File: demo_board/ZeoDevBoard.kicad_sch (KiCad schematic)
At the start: 0 parts

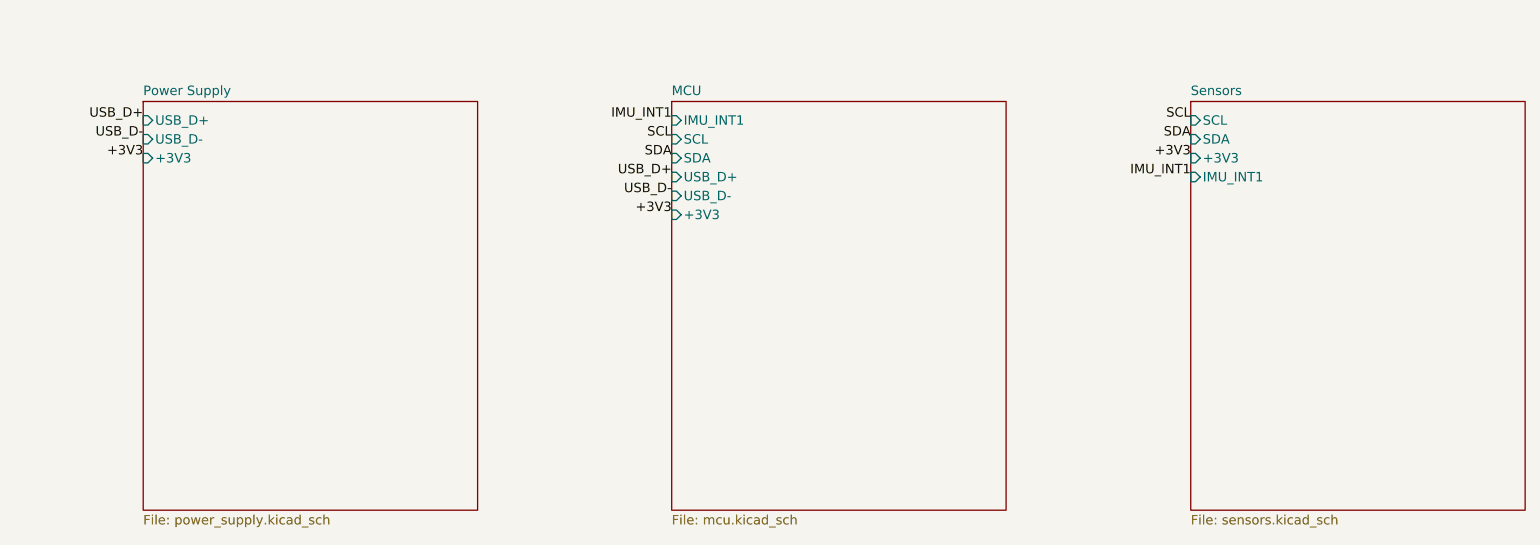
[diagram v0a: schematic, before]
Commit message: new demo board
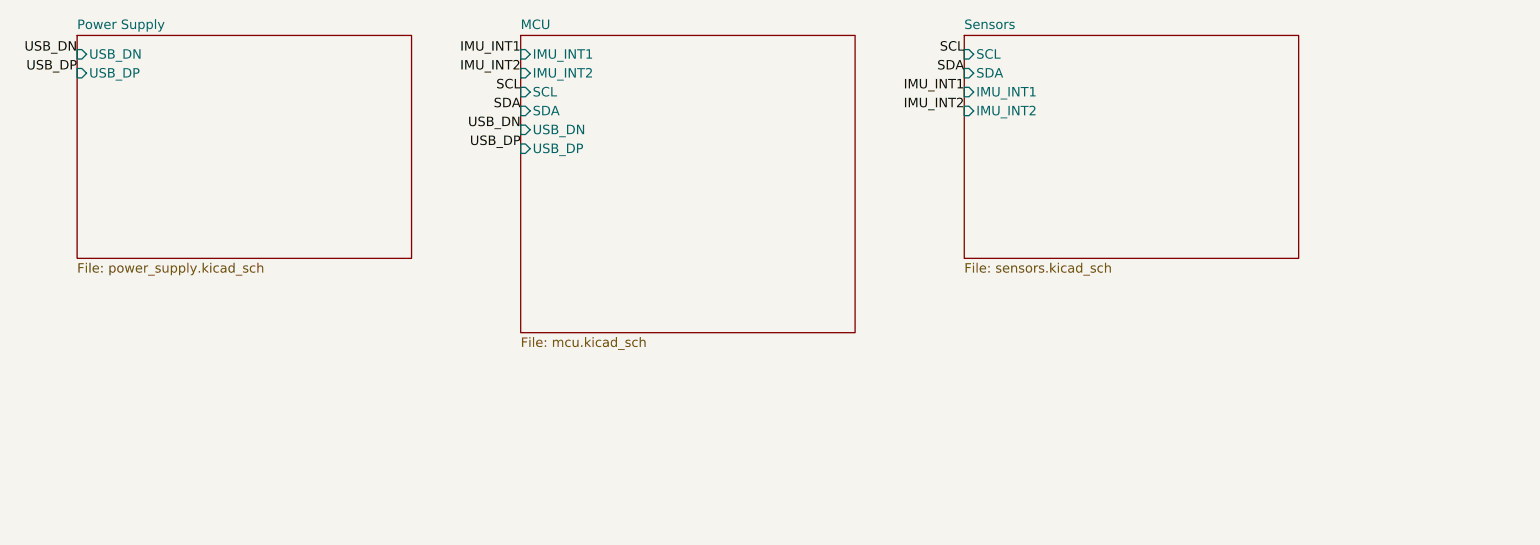
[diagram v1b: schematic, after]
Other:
- sheet MCU ports: added IMU_INT2, USB_DN, USB_DP; removed +3V3, USB_D+, USB_D-
- sheet Power Supply ports: added USB_DN, USB_DP; removed +3V3, USB_D+, USB_D-
- sheet Sensors ports: added IMU_INT2; removed +3V3
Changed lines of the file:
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@@
 	(generator_version "10.0")
 	(paper "A4")
-	(label "USB_D-"
-		(at 39.37 44.45 180)
-		(effects
-			(font
-				(size 1.27 1.27)
-				(line_spacing 0)
-			)
-			(justify right bottom)
-		)
-	)
-	(label "+3V3"
-		(at 110.49 54.61 180)
+	(label "USB_DP"
+		(at 30.48 35.56 180)
+		(effects
+			(font
+				(size 1.27 1.27)
+				(line_spacing 0)
+			)
+			(justify right bottom)
+		)
+	)
+	(label "IMU_INT2"
+		(at 90.17 35.56 180)
+		(effects
+			(font
+				(size 1.27 1.27)
+				(line_spacing 0)
+			)
+			(justify right bottom)
+		)
+	)
+	(label "USB_DN"
+		(at 30.48 33.02 180)
+		(effects
+			(font
+				(size 1.27 1.27)
+				(line_spacing 0)
+			)
+			(justify right bottom)
+		)
+	)
+	(label "USB_DP"
+		(at 90.17 45.72 180)
+		(effects
+			(font
+				(size 1.27 1.27)
+				(line_spacing 0)
+			)
+			(justify right bottom)
+		)
+	)
+	(label "IMU_INT1"
+		(at 149.86 38.1 180)
+		(effects
+			(font
+				(size 1.27 1.27)
+				(line_spacing 0)
+			)
+			(justify right bottom)
+		)
+	)
+	(label "USB_DN"
+		(at 90.17 43.18 180)
+		(effects
+			(font
+				(size 1.27 1.27)
+				(line_spacing 0)
+			)
+			(justify right bottom)
+		)
+	)
+	(label "IMU_INT2"
+		(at 149.86 40.64 180)
 		(effects
 			(font
@@
 	)
 	(label "SCL"
-		(at 110.49 44.45 180)
-		(effects
-			(font
-				(size 1.27 1.27)
-				(line_spacing 0)
-			)
-			(justify right bottom)
-		)
-	)
-	(label "USB_D+"
-		(at 39.37 41.91 180)
+		(at 149.86 33.02 180)
+		(effects
+			(font
+				(size 1.27 1.27)
+				(line_spacing 0)
+			)
+			(justify right bottom)
+		)
+	)
+	(label "SCL"
+		(at 90.17 38.1 180)
+		(effects
+			(font
+				(size 1.27 1.27)
+				(line_spacing 0)
+			)
+			(justify right bottom)
+		)
+	)
+	(label "SDA"
+		(at 90.17 40.64 180)
 		(effects
 			(font
@@
 	)
 	(label "IMU_INT1"
-		(at 180.34 49.53 180)
+		(at 90.17 33.02 180)
 		(effects
 			(font
@@
 	)
 	(label "SDA"
-		(at 180.34 44.45 180)
-		(effects
-			(font
-				(size 1.27 1.27)
-				(line_spacing 0)
-			)
-			(justify right bottom)
-		)
-	)
-	(label "+3V3"
-		(at 39.37 46.99 180)
-		(effects
-			(font
-				(size 1.27 1.27)
-				(line_spacing 0)
-			)
-			(justify right bottom)
-		)
-	)
-	(label "+3V3"
-		(at 180.34 46.99 180)
-		(effects
-			(font
-				(size 1.27 1.27)
-				(line_spacing 0)
-			)
-			(justify right bottom)
-		)
-	)
-	(label "SCL"
-		(at 180.34 41.91 180)
-		(effects
-			(font
-				(size 1.27 1.27)
-				(line_spacing 0)
-			)
-			(justify right bottom)
-		)
-	)
-	(label "USB_D+"
-		(at 110.49 49.53 180)
-		(effects
-			(font
-				(size 1.27 1.27)
-				(line_spacing 0)
-			)
-			(justify right bottom)
-		)
-	)
-	(label "SDA"
-		(at 110.49 46.99 180)
-		(effects
-			(font
-				(size 1.27 1.27)
-				(line_spacing 0)
-			)
-			(justify right bottom)
-		)
-	)
-	(label "USB_D-"
-		(at 110.49 52.07 180)
-		(effects
-			(font
-				(size 1.27 1.27)
-				(line_spacing 0)
-			)
-			(justify right bottom)
-		)
-	)
-	(label "IMU_INT1"
-		(at 110.49 41.91 180)
+		(at 149.86 35.56 180)
 		(effects
 			(font
@@
 	)
 	(sheet
-		(at 180.34 39.37)
-		(size 45 55)
+		(at 149.86 30.48)
+		(size 45 30)
 		(exclude_from_sim no)
 		(in_bom yes)
@@
 		)
 		(property "Sheetname" "Sensors"
-			(at 180.34 38.6584 0)
+			(at 149.86 29.7684 0)
 			(show_name no)
 			(do_not_autoplace no)
@@
 		)
 		(property "Sheetfile" "sensors.kicad_sch"
-			(at 180.34 94.9546 0)
+			(at 149.86 61.0646 0)
 			(show_name no)
 			(do_not_autoplace no)
@@
 		)
 		(pin "SCL" input
-			(at 180.34 41.91 180)
+			(at 149.86 33.02 180)
 			(effects
 				(font
@@
 		)
 		(pin "SDA" input
-			(at 180.34 44.45 180)
-			(effects
-				(font
-					(size 1.27 1.27)
-				)
-				(justify left)
-			)
-		)
-		(pin "+3V3" input
-			(at 180.34 46.99 180)
+			(at 149.86 35.56 180)
 			(effects
 				(font
@@
 		)
 		(pin "IMU_INT1" input
-			(at 180.34 49.53 180)
+			(at 149.86 38.1 180)
+			(effects
+				(font
+					(size 1.27 1.27)
+				)
+				(justify left)
+			)
+		)
+		(pin "IMU_INT2" input
+			(at 149.86 40.64 180)
 			(effects
 				(font
@@
 	)
 	(sheet
-		(at 110.49 39.37)
-		(size 45 55)
+		(at 30.48 30.48)
+		(size 45 30)
 		(exclude_from_sim no)
 		(in_bom yes)
@@
 			(color 0 0 0 0)
 		)
-		(property "Sheetname" "MCU"
-			(at 110.49 38.6584 0)
+		(property "Sheetname" "Power Supply"
+			(at 30.48 29.7684 0)
 			(show_name no)
 			(do_not_autoplace no)
@@
 			)
 		)
-		(property "Sheetfile" "mcu.kicad_sch"
-			(at 110.49 94.9546 0)
+		(property "Sheetfile" "power_supply.kicad_sch"
+			(at 30.48 61.0646 0)
 			(show_name no)
 			(do_not_autoplace no)
@@
 			)
 		)
-		(pin "IMU_INT1" input
-			(at 110.49 41.91 180)
-			(effects
-				(font
-					(size 1.27 1.27)
-				)
-				(justify left)
-			)
-		)
-		(pin "SCL" input
-			(at 110.49 44.45 180)
-			(effects
-				(font
-					(size 1.27 1.27)
-				)
-				(justify left)
-			)
-		)
-		(pin "SDA" input
-			(at 110.49 46.99 180)
-			(effects
-				(font
-					(size 1.27 1.27)
-				)
-				(justify left)
-			)
-		)
-		(pin "USB_D+" input
-			(at 110.49 49.53 180)
-			(effects
-				(font
-					(size 1.27 1.27)
-				)
-				(justify left)
-			)
-		)
-		(pin "USB_D-" input
-			(at 110.49 52.07 180)
-			(effects
-				(font
-					(size 1.27 1.27)
-				)
-				(justify left)
-			)
-		)
-		(pin "+3V3" input
-			(at 110.49 54.61 180)
+		(pin "USB_DN" input
+			(at 30.48 33.02 180)
+			(effects
+				(font
+					(size 1.27 1.27)
+				)
+				(justify left)
+			)
+		)
+		(pin "USB_DP" input
+			(at 30.48 35.56 180)
 			(effects
 				(font
@@
 	)
 	(sheet
-		(at 39.37 39.37)
-		(size 45 55)
+		(at 90.17 30.48)
+		(size 45 40)
 		(exclude_from_sim no)
 		(in_bom yes)
@@
 			(color 0 0 0 0)
 		)
-		(property "Sheetname" "Power Supply"
-			(at 39.37 38.6584 0)
+		(property "Sheetname" "MCU"
+			(at 90.17 29.7684 0)
 			(show_name no)
 			(do_not_autoplace no)
@@
 			)
 		)
-		(property "Sheetfile" "power_supply.kicad_sch"
-			(at 39.37 94.9546 0)
+		(property "Sheetfile" "mcu.kicad_sch"
+			(at 90.17 71.0646 0)
 			(show_name no)
 			(do_not_autoplace no)
@@
 			)
 		)
-		(pin "USB_D+" input
-			(at 39.37 41.91 180)
-			(effects
-				(font
-					(size 1.27 1.27)
-				)
-				(justify left)
-			)
-		)
-		(pin "USB_D-" input
-			(at 39.37 44.45 180)
-			(effects
-				(font
-					(size 1.27 1.27)
-				)
-				(justify left)
-			)
-		)
-		(pin "+3V3" input
-			(at 39.37 46.99 180)
-			(effects
-				(font
+		(pin "IMU_INT1" input
+			(at 90.17 33.02 180)
+			(effects
+				(font
+					(size 1.27 1.27)
+				)
+				(justify left)
+			)
+		)
+		(pin "IMU_INT2" input
+			(at 90.17 35.56 180)
+			(effects
+				(font
+					(size 1.27 1.27)
+				)
+				(justify left)
+			)
+		)
+		(pin "SCL" input
+			(at 90.17 38.1 180)
+			(effects
+				(font
+					(size 1.27 1.27)
+				)
+				(justify left)
+			)
+		)
+		(pin "SDA" input
+			(at 90.17 40.64 180)
+			(effects
+				(font
+					(size 1.27 1.27)
+				)
+				(justify left)
+			)
+		)
+		(pin "USB_DN" input
+			(at 90.17 43.18 180)
+			(effects
+				(font
+					(size 1.27 1.27)
+				)
+				(justify left)
+			)
+		)
+		(pin "USB_DP" input
+			(at 90.17 45.72 180)
+			(effects
+				(font
